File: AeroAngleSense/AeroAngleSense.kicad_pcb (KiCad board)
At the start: 2 copper layers, 15 x 55 mm, 23 parts, among them IC1 STM32F042F6P6, IC2 TMP127EDBVRQ1, IC3 TPS62842DGRR, J1 SM06B-GHS-TBT, J7 SM04B-GHS-TBT

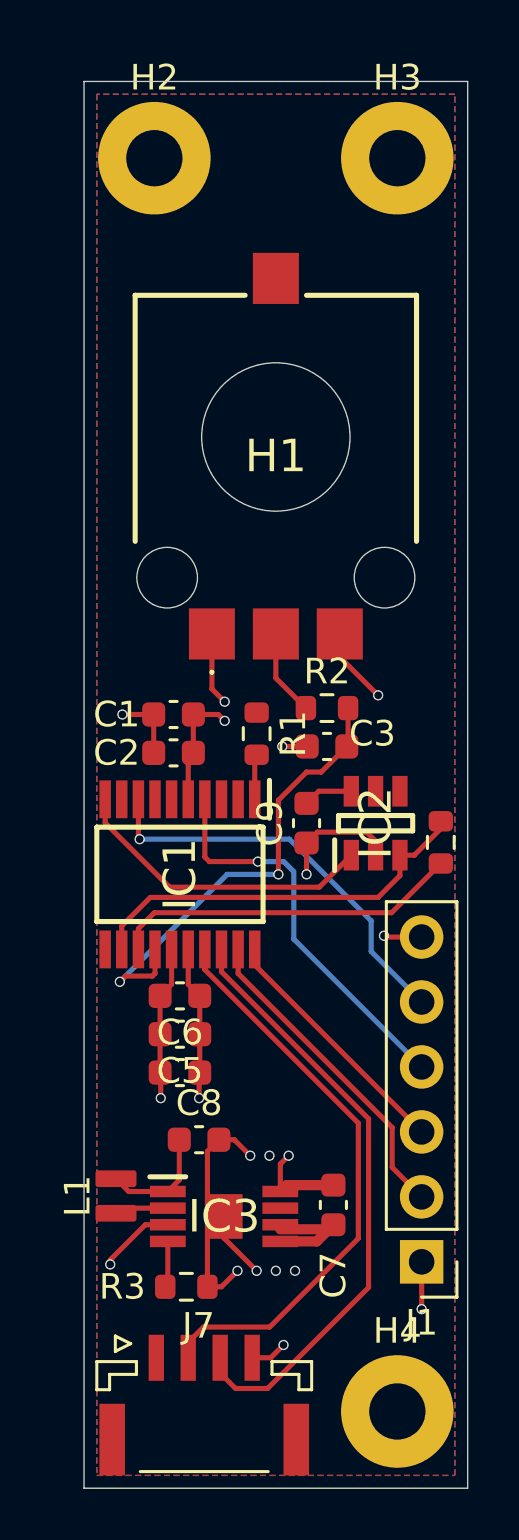
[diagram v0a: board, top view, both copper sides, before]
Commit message: 배선_3
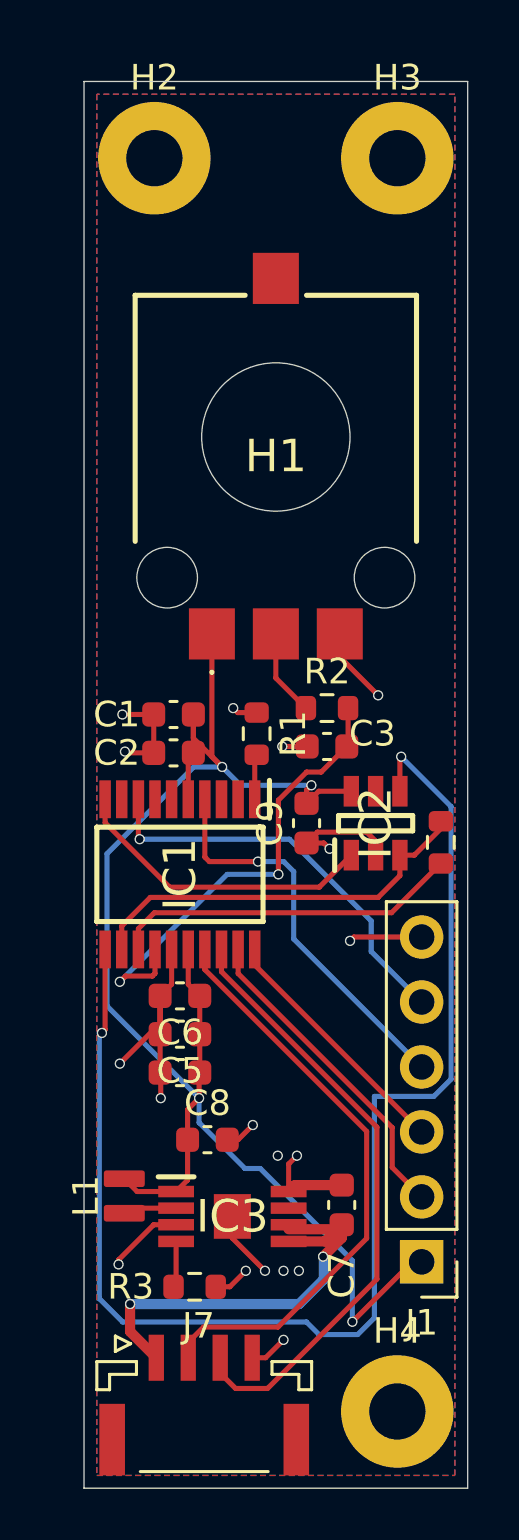
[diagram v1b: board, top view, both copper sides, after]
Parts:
- moved C7 0.32 mm to (30.1, 58.9)
- moved C8 0.32 mm to (24.8, 56.4)
- moved IC3 0.32 mm to (25.8, 59.4)
- moved L1 0.32 mm to (21.6, 58.6)
- moved R3 0.32 mm to (24.3, 62.1)
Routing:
- net /TMP_SCLK: track 0.00 -> 52.1 mm, vias 0 -> 2
- net +3.3V: track 21.8 -> 62.6 mm
- net +5V: track 4.49 -> 17.4 mm, vias 0 -> 2
- net GND: track 38.7 -> 39.1 mm, vias 15 -> 18
